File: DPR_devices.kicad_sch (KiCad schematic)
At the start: 31 parts, among them J10 M12_P2, J11 SMA_P3, J6 M12_P1, J7 M12_P3, J8 SMA_P1, J9 SMA_P2, U10 PCA9548APW, U7 ADS8681IPW, U8 ADS8681IPW, U9 ADS8681IPW

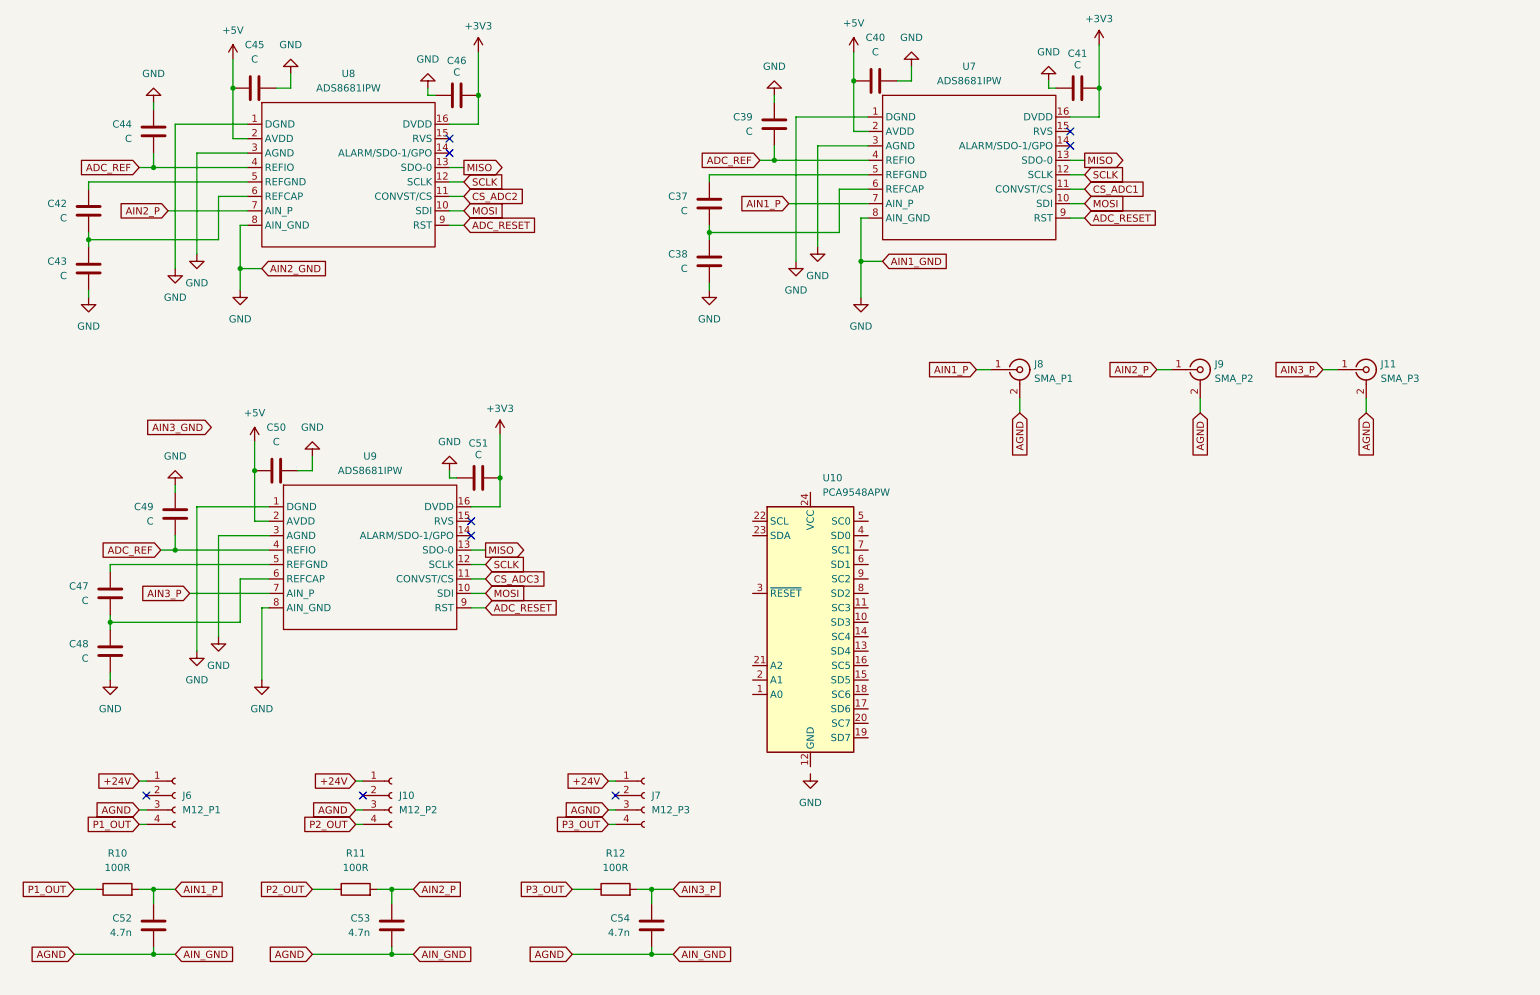
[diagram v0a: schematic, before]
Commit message: Schematic ok (je crois)
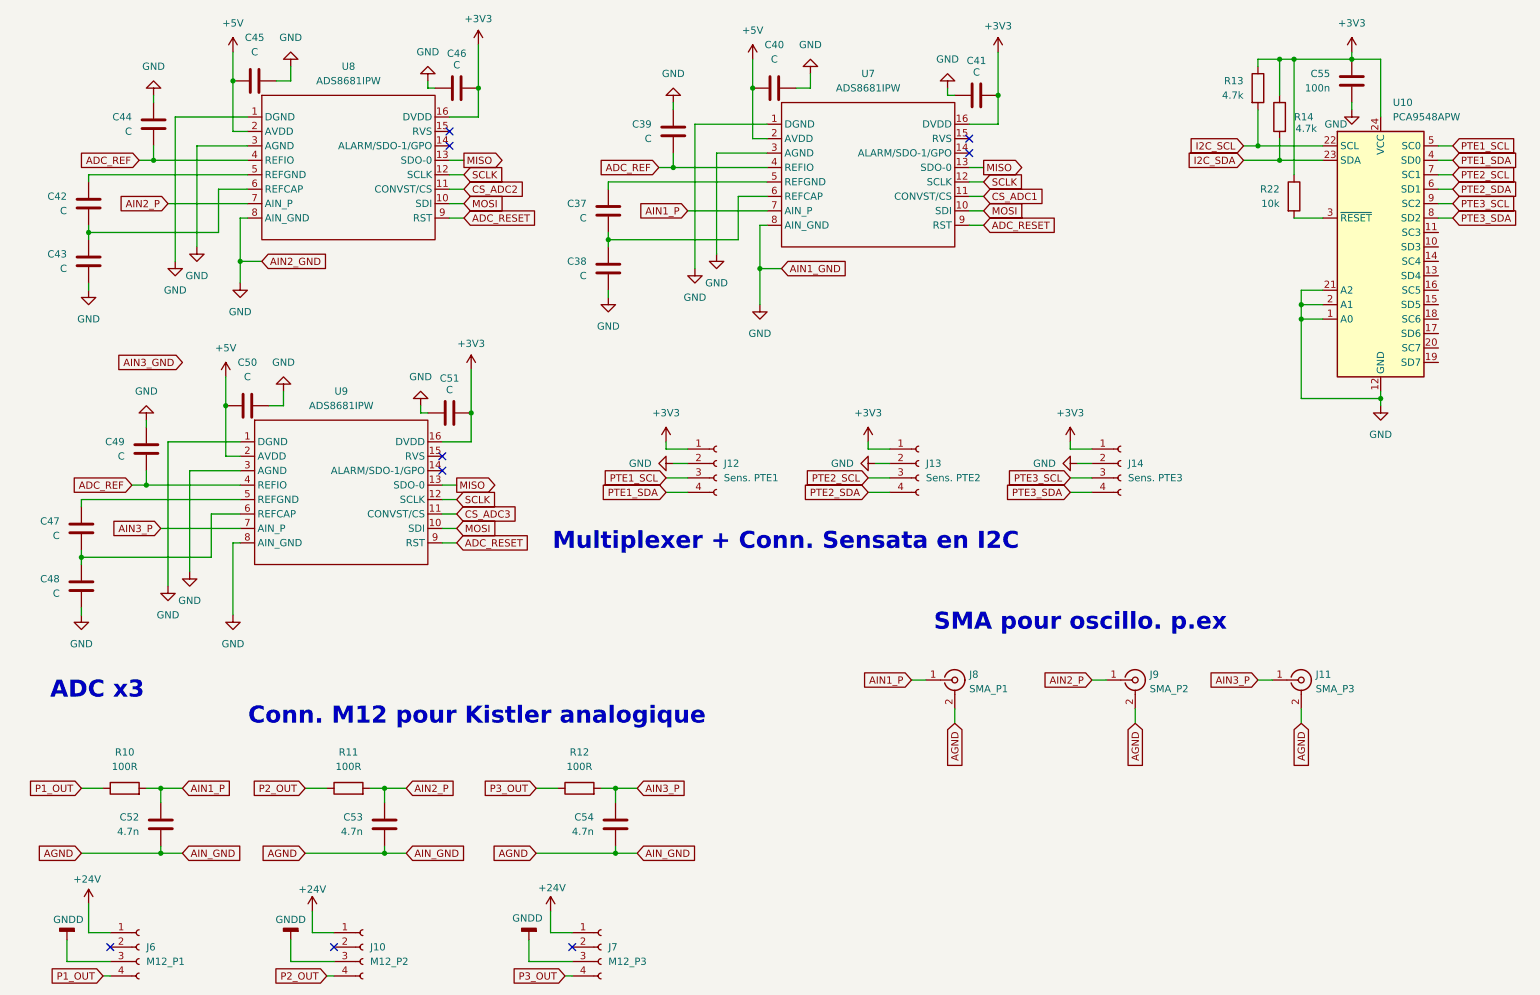
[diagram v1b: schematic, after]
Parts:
- added C55: 100n, symbol Device:C
- added J12: Sens. PTE1, symbol Connector:Conn_01x04_Socket
- added J13: Sens. PTE2, symbol Connector:Conn_01x04_Socket
- added J14: Sens. PTE3, symbol Connector:Conn_01x04_Socket
- added R13, R14: 4.7k, symbol DPR_devices:R
- added R22: 10k, symbol DPR_devices:R
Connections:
- net +3V3: now also U10.24 (VCC), C55.2, J12.1 (Pin_1), J13.1 (Pin_1), J14.1 (Pin_1), R13.1, R14.1, R22.1
- net AGND: no longer J10.3 (Pin_3), J6.3 (Pin_3), J7.3 (Pin_3)
- net GND: now also U10.1 (A0), U10.12 (GND), U10.2 (A1), U10.21 (A2), C55.1, J12.2 (Pin_2), J13.2 (Pin_2), J14.2 (Pin_2)
- net I2C_SCL: now reaches U10.22 (SCL)
- net I2C_SCL: now also R13.2
- net I2C_SDA: now reaches U10.23 (SDA)
- net I2C_SDA: now also R14.2
- net at U10.3 (~{RESET}): now also R22.2
- net PTE1_SDA: now reaches U10.4 (SD0)
- net PTE1_SDA: now also J12.4 (Pin_4)
- net PTE1_SCL: now reaches U10.5 (SC0)
- net PTE1_SCL: now also J12.3 (Pin_3)
- net PTE2_SDA: now reaches U10.6 (SD1)
- net PTE2_SDA: now also J13.4 (Pin_4)
- net PTE2_SCL: now reaches U10.7 (SC1)
- net PTE2_SCL: now also J13.3 (Pin_3)
- net PTE3_SDA: now reaches U10.8 (SD2)
- net PTE3_SDA: now also J14.4 (Pin_4)
- net PTE3_SCL: now reaches U10.9 (SC2)
- net PTE3_SCL: now also J14.3 (Pin_3)
- new net GNDD: J10.3 (Pin_3), J6.3 (Pin_3), J7.3 (Pin_3)
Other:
- note added: "ADC x3"
- note added: "Conn. M12 pour Kistler analogique"
- note added: "Multiplexer + Conn. Sensata en I2C"
- note added: "SMA pour oscillo. p.ex"
- moved on the sheet: C37, C38, C39, C40, C41, C42, C43, C44, C45, C46, C47, C48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
